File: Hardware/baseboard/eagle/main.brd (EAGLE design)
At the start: 169.7 x 96 mm, 173 parts, among them X1 JST-4POS-2X4POS, X1.2 TACH/LAP, X2 ATLAS-LTC, X2.1 MOTOR, X2.2 VRAILS+, X2.3 5V+SoC, X4 SYSTEWI, X5 15244441

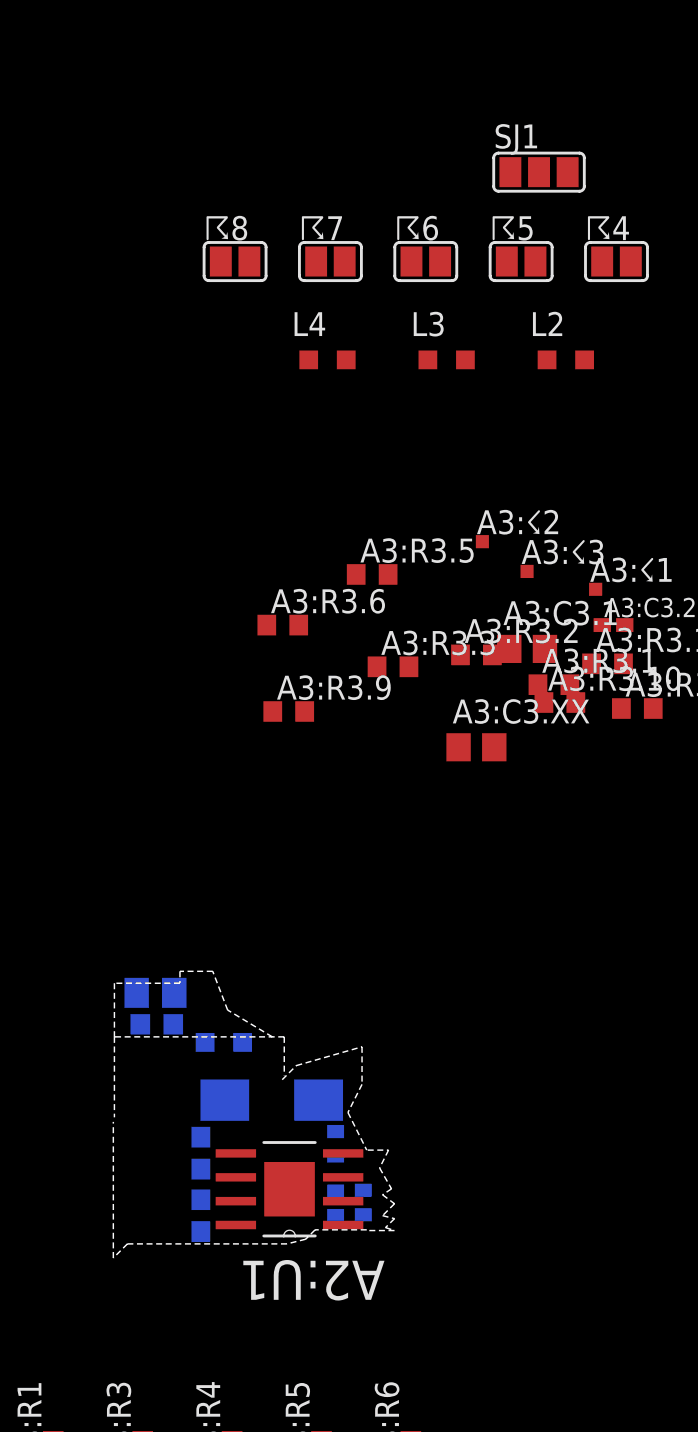
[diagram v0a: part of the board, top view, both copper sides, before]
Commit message: wip baseboard qucksave  + placement for motor driver good enough  + touchdown now into baseboard  + everything's fine
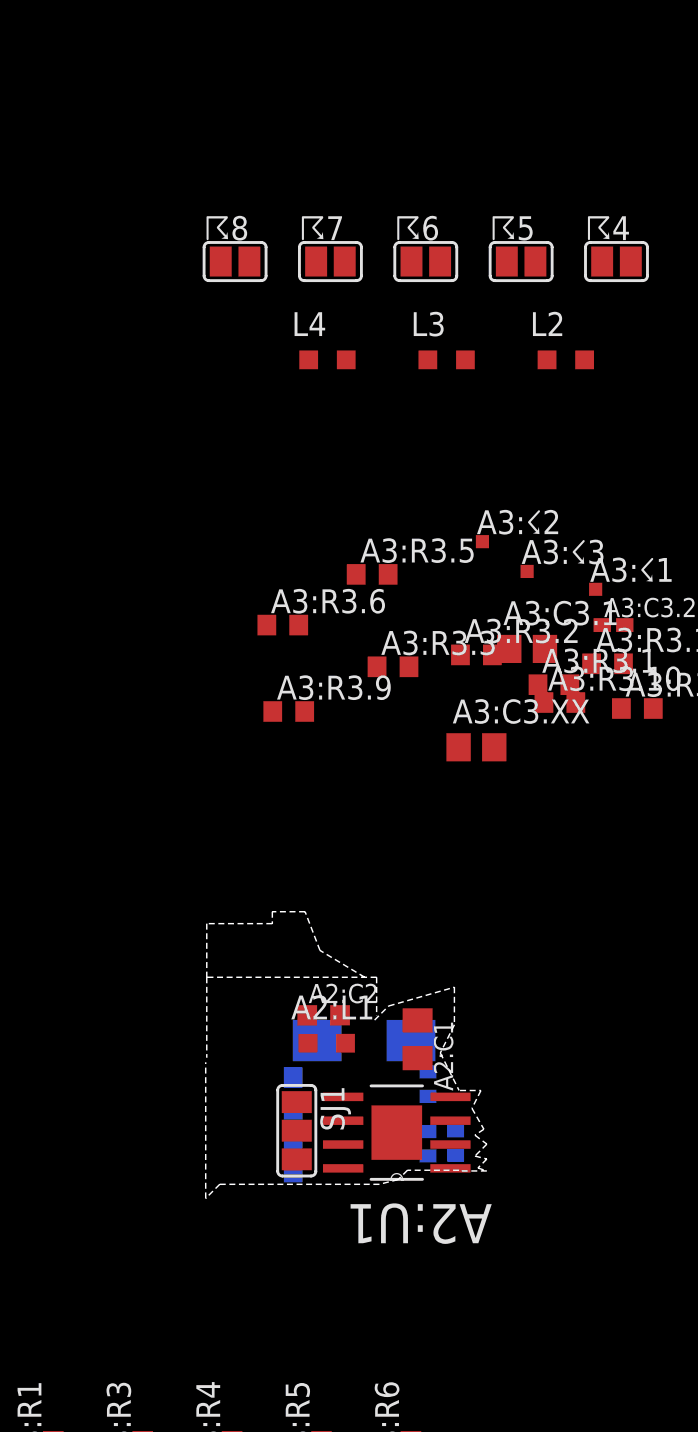
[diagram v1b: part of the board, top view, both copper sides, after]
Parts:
- moved SJ1 52.7 mm to (120.5, 44.5), turned to 270 degrees
- moved A2:C1 14.2 mm to (127.0, 49.4), flipped to the top, turned to 270 degrees
- moved A2:C2 8.90 mm to (122.0, 50.7), flipped to the top
- moved A2:U1 6.46 mm to (125.9, 44.4)
- moved A2:R3 5.86 mm to (129.0, 43.9)
- moved A2:C3 5.86 mm to (124.1, 49.3)
- moved A2:C4 5.86 mm to (120.3, 46.5)
- moved A2:C5 5.86 mm to (120.3, 43.2)
- moved A2:R1 5.86 mm to (127.5, 47.0)
- moved A2:R2 5.86 mm to (127.5, 43.8)
- moved A2:L1 5.49 mm to (122.1, 49.2), flipped to the top, turned to 0 degrees
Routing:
- net GND: track 27.3 -> 26.3 mm
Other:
- board size 169.7 x 96 mm -> 174.7 x 97.2 mm
